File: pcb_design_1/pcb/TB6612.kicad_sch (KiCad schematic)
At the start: 6 parts, among them J3 Conn_01x08_Socket, J4 Conn_01x08_Socket, J5 Conn_01x08_Pin, J6 Conn_01x08_Pin, U4 TB6612FNG

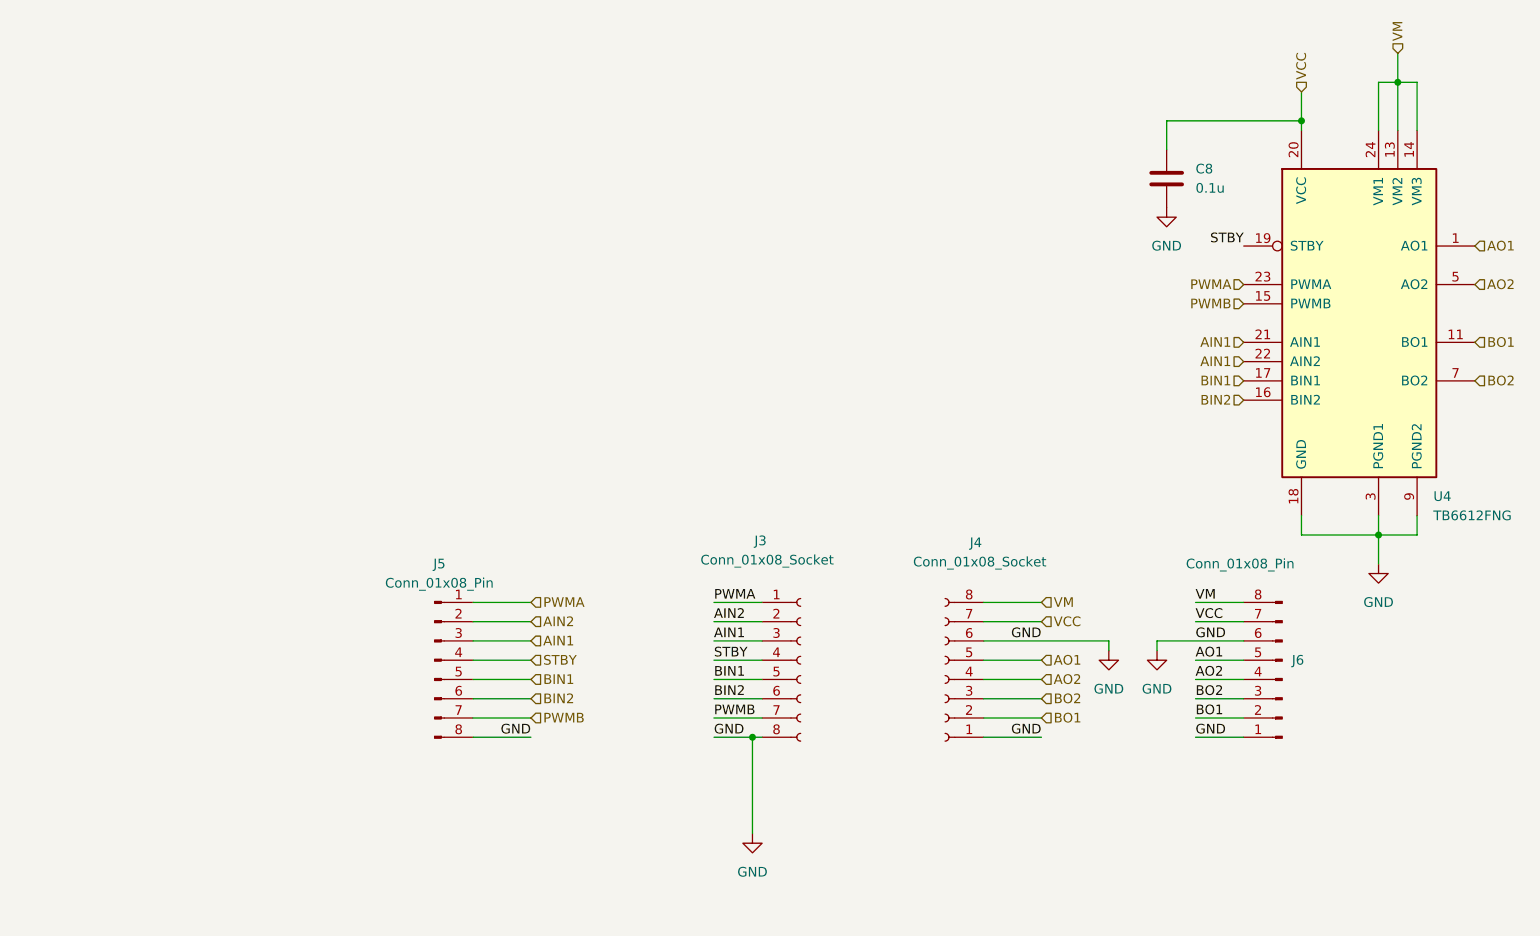
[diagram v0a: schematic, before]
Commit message: improved the designed
improved the designed
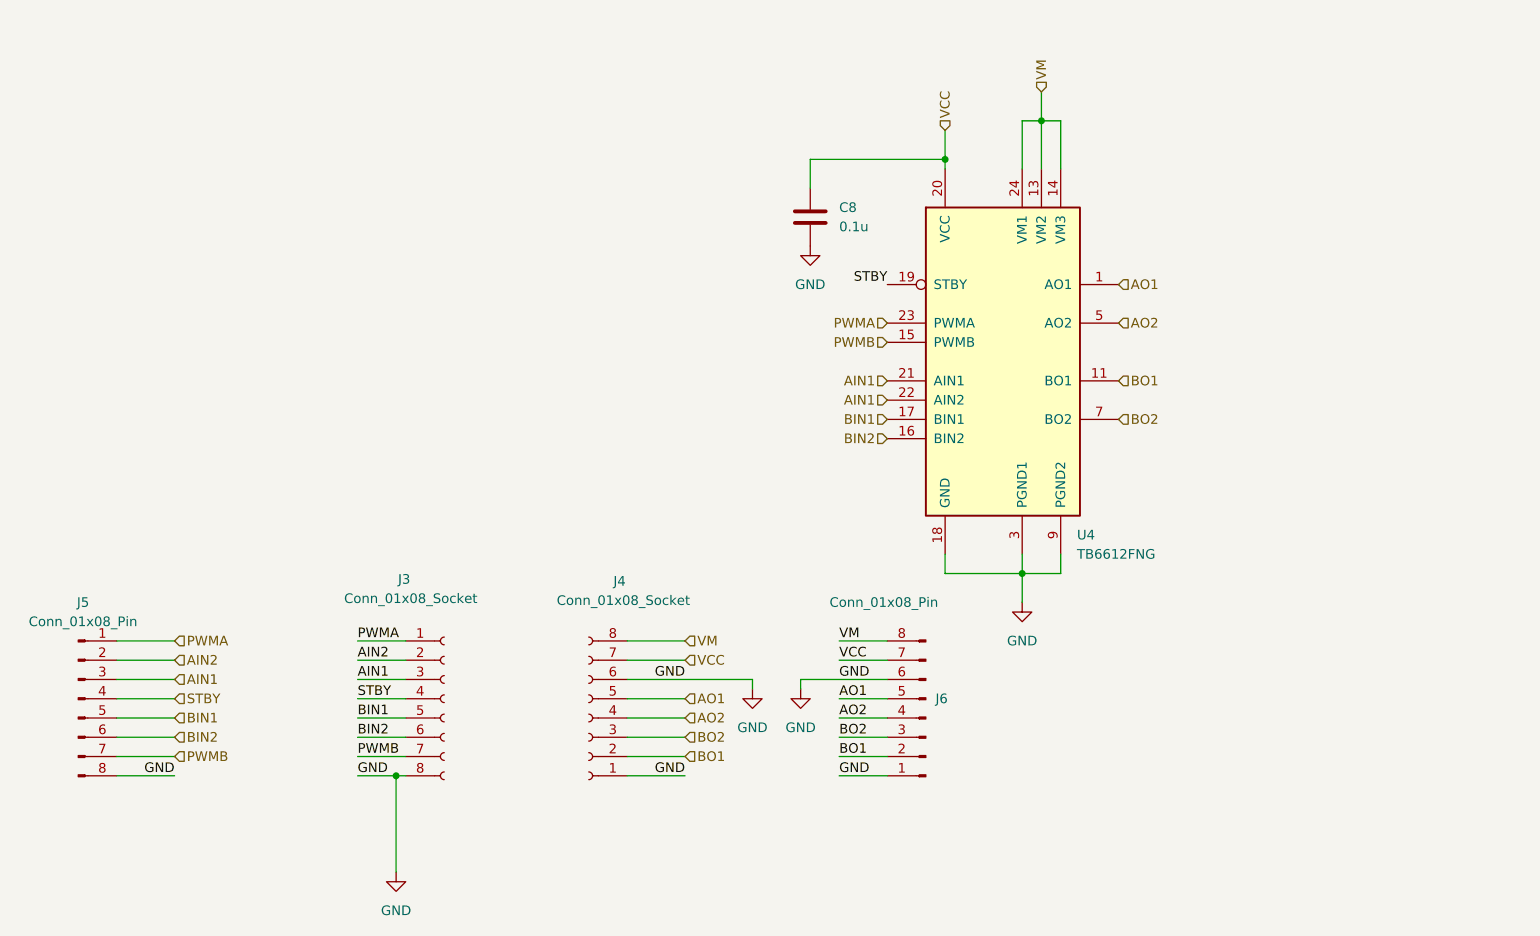
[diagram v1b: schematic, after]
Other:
- moved on the sheet: C8, J3, J4, J5, J6, U4
